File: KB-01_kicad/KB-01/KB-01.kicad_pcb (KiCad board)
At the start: 6 copper layers, 80 x 120 mm, 138 parts, among them IC1 MAX17048G+T10, J1 Conn_01x22_MountingPin, J11 Conn_02x07_Odd_Even, J12 Conn_01x01_Socket, J13 Conn_01x22_MountingPin, J14 Micro_SD_Card_Det, J15 Conn_Coaxial, J3 USB_C_Receptacle_USB2.0_14P, J4 Conn_01x02_MountingPin, J5 Conn_01x01_Socket, J8 Bus_M.2_Socket_M, J9 AudioJack3_SwitchTR, Q1 MMBT3904, Q2 2N7002, SW1 Right angle Tact button, SW2 Power button, SW3 RotaryEncoder_Switch_MP, SW4 SW_Push, SW5 SW_Push, U1 BQ25895, U10 AP3441SHE-7B, U11 BMP581, U12 BMI270, U13 SHT40, U14 LIS2MDL, U18 RT9742GGJ5 / NCP380HSN10AAT1G, U2 TS3USB30ERSWR, U3 TLV70430DBVR, U4 TPS61022, U5 TLV773_SOT353, U6 TESEO-LIV4F, U9 ASEK-32.768KHZ-L-R-T

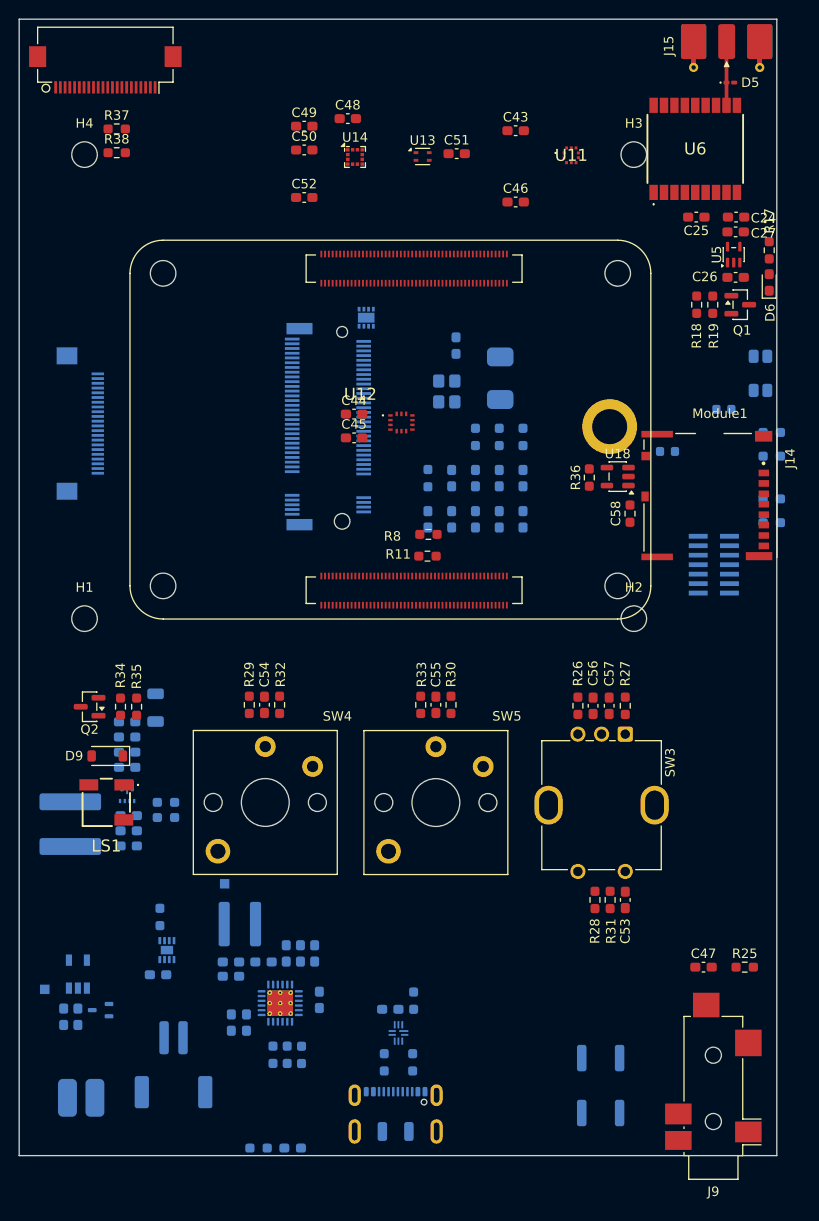
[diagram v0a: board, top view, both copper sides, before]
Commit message: all
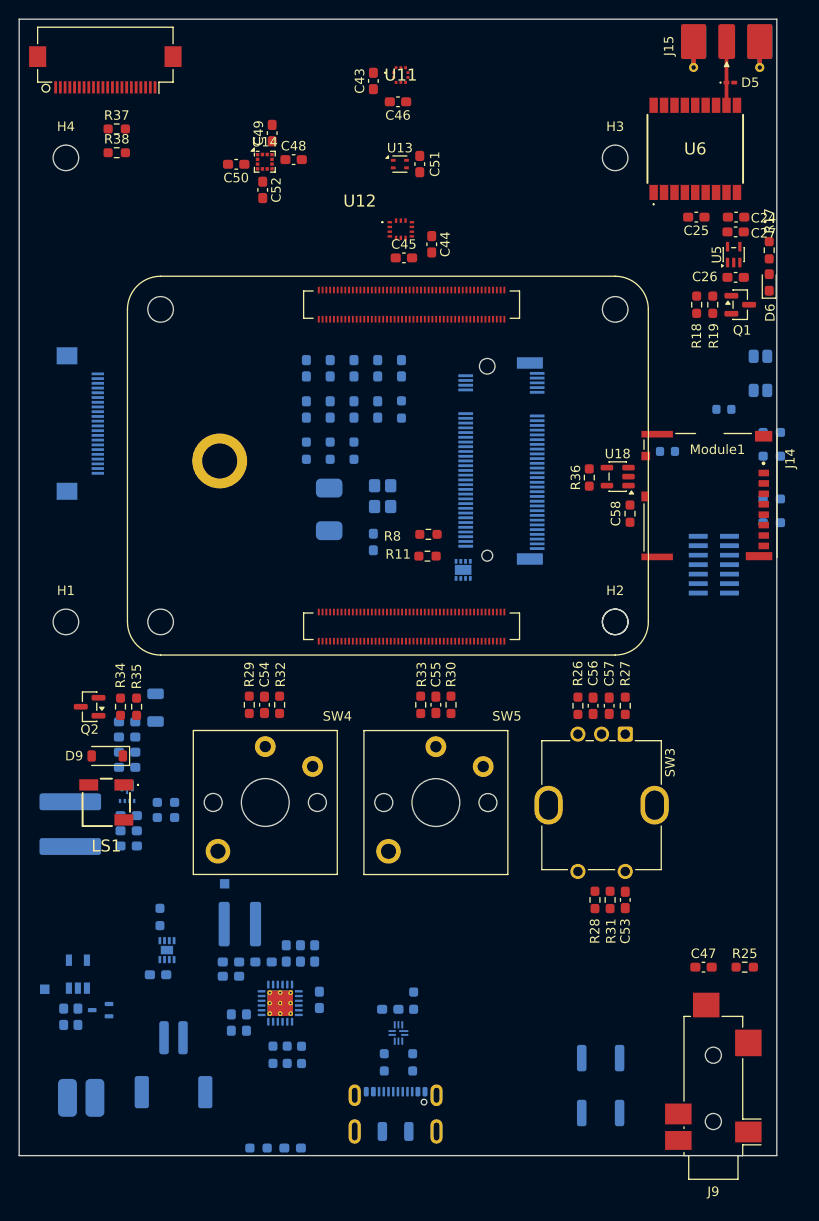
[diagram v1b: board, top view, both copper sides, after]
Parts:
- moved U10 28.5 mm to (110.5, 94.9), turned to -90 degrees
- moved C34 27.9 mm to (93.9, 73.6), turned to -90 degrees
- moved C39 24.0 mm to (93.9, 77.9), turned to -90 degrees
- moved C35 23.9 mm to (96.4, 73.6), turned to -90 degrees
- moved R22 22.9 mm to (93.9, 82.3), turned to -90 degrees
- moved L5 22.8 mm to (96.3, 88.5), turned to -90 degrees
- moved D8 22.5 mm to (101.0, 91.9), turned to -90 degrees
- moved C36 20.5 mm to (98.9, 73.6), turned to -90 degrees
- moved U12 20.4 mm to (103.9, 58.9)
- moved U11 19.9 mm to (103.9, 42.6)
- moved C45 19.7 mm to (104.2, 61.9)
- moved C44 19.7 mm to (107.2, 60.5), turned to -90 degrees
- moved C40 19.3 mm to (96.4, 77.9), turned to -90 degrees
- moved R23 17.9 mm to (96.4, 82.3), turned to -90 degrees
- moved C37 17.8 mm to (101.5, 73.6), turned to -90 degrees
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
